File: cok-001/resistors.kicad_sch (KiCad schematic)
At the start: 90 parts, among them Q1101 DTC144E, Q1102 DTC144E, U1101 ADT7461A0002RMZR

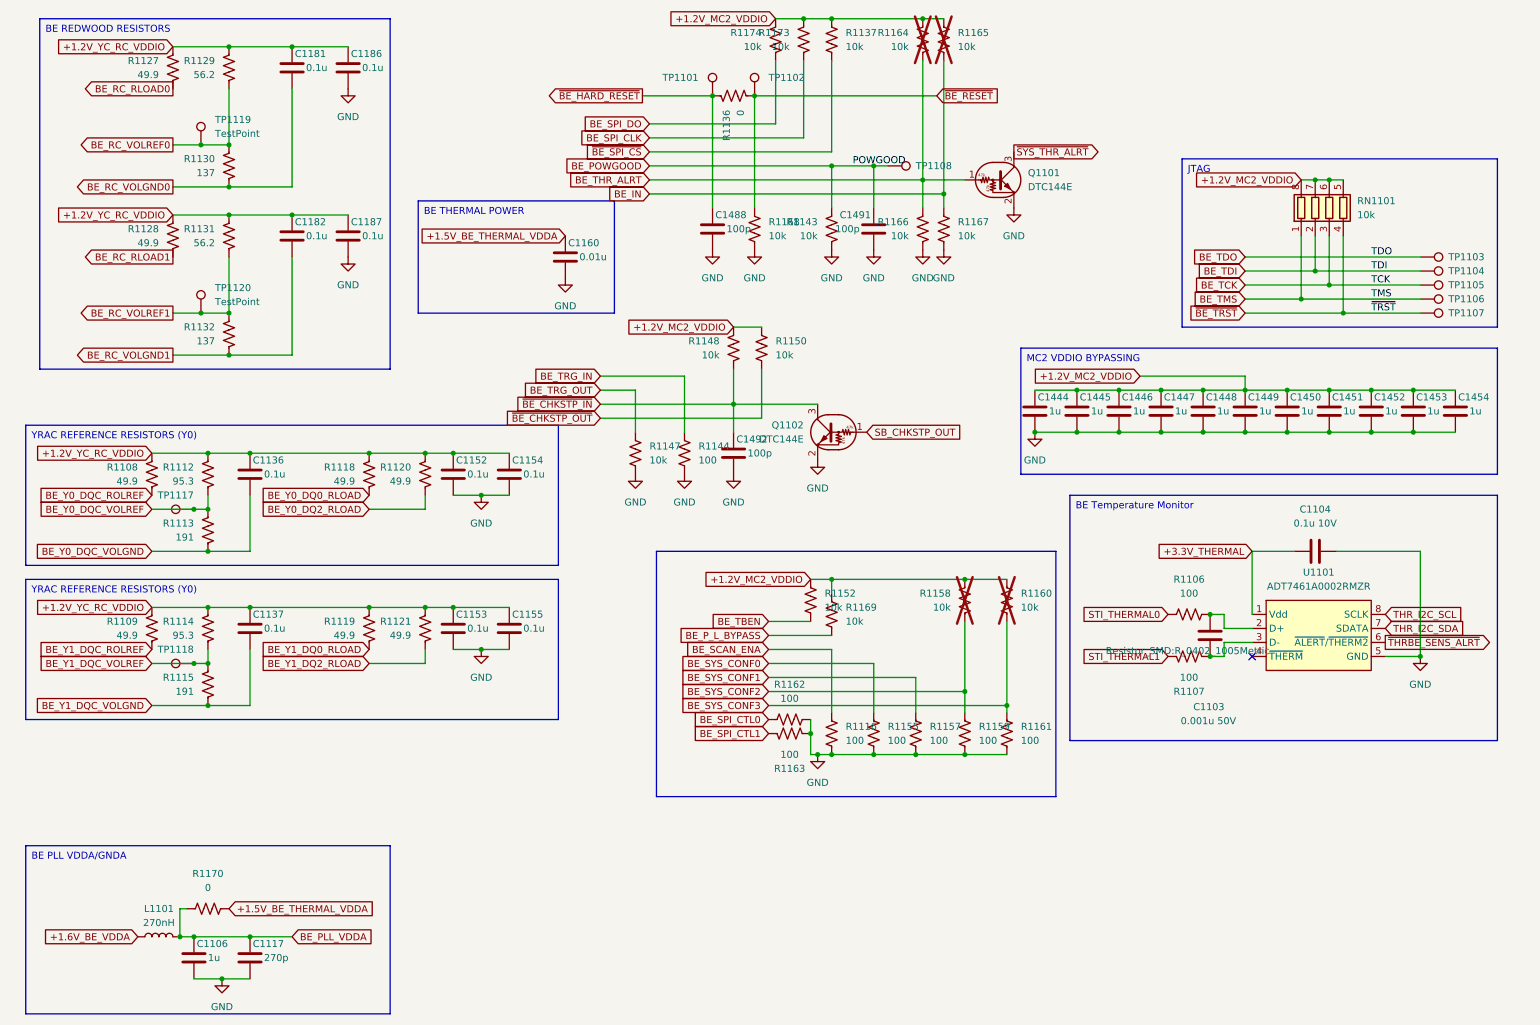
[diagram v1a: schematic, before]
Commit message: update to 9
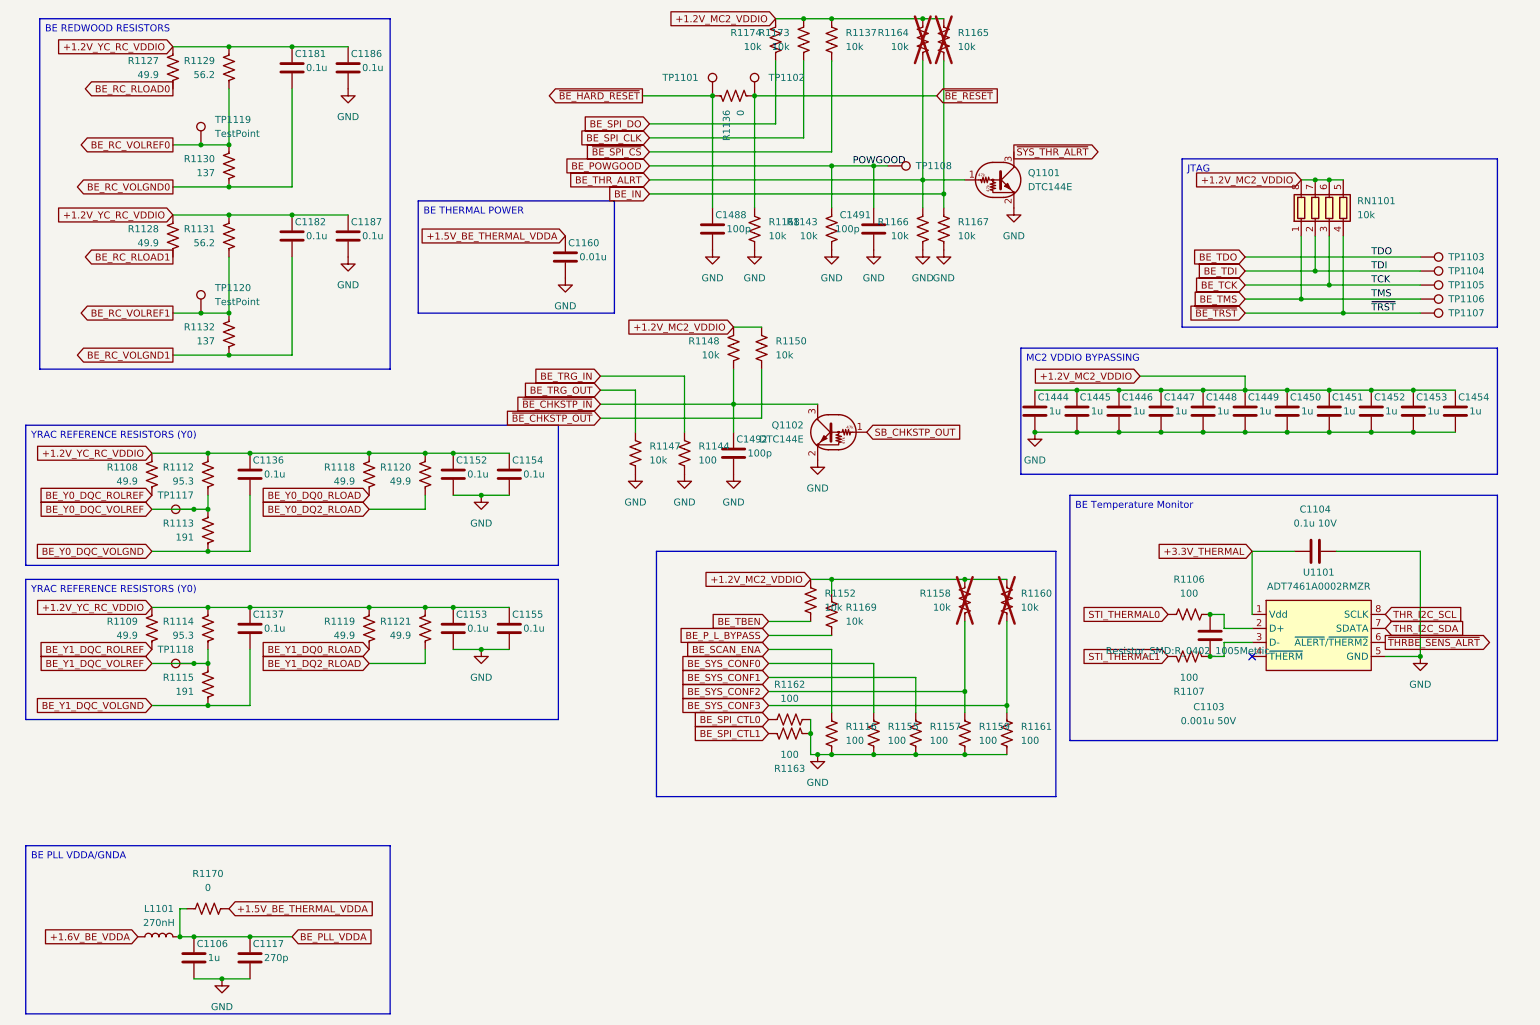
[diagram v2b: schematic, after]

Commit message: msop
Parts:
- U1101: footprint Package_SO:MSOP-8_3x3mm_P0.65mm -> PS3:MSOP-8_2.9x4mm_P0.65mm
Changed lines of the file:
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@@
 			)
 		)
-		(property "Footprint" "Package_SO:MSOP-8_3x3mm_P0.65mm"
+		(property "Footprint" "PS3:MSOP-8_2.9x4mm_P0.65mm"
 			(at 250.19 119.38 0)
 			(effects
